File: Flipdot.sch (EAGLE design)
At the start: 20 parts, among them IC1 ULN2003, IC10 ULN2003, IC11 M74HC238, IC12 M74HC238, IC13 M74HC238, IC14 TD62783_AFWG, IC15 ULN2003, IC16 TD62783_AFWG, IC17 ULN2003, IC18 M74HC238, IC2 TD62783_AFWG, IC3 M74HC238, IC4 M74HC238, IC5 M74HC238, IC6 M74HC238, IC7 TD62783_AFWG, IC8 ULN2003, IC9 TD62783_AFWG, J1 HEADER

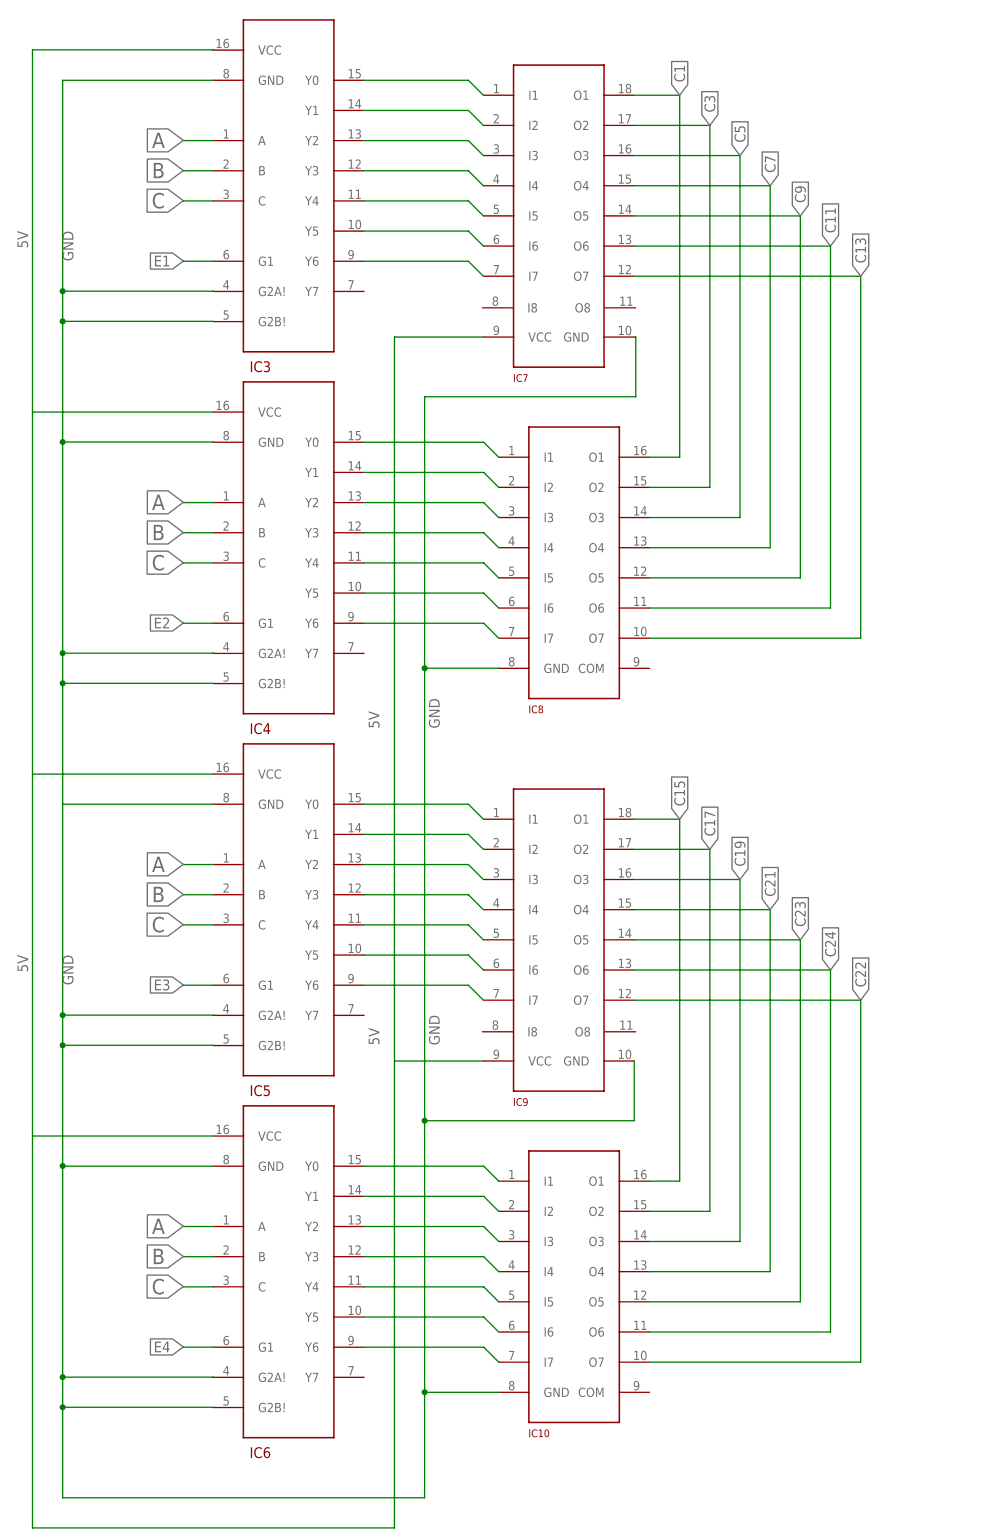
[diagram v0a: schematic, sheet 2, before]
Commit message: Finished
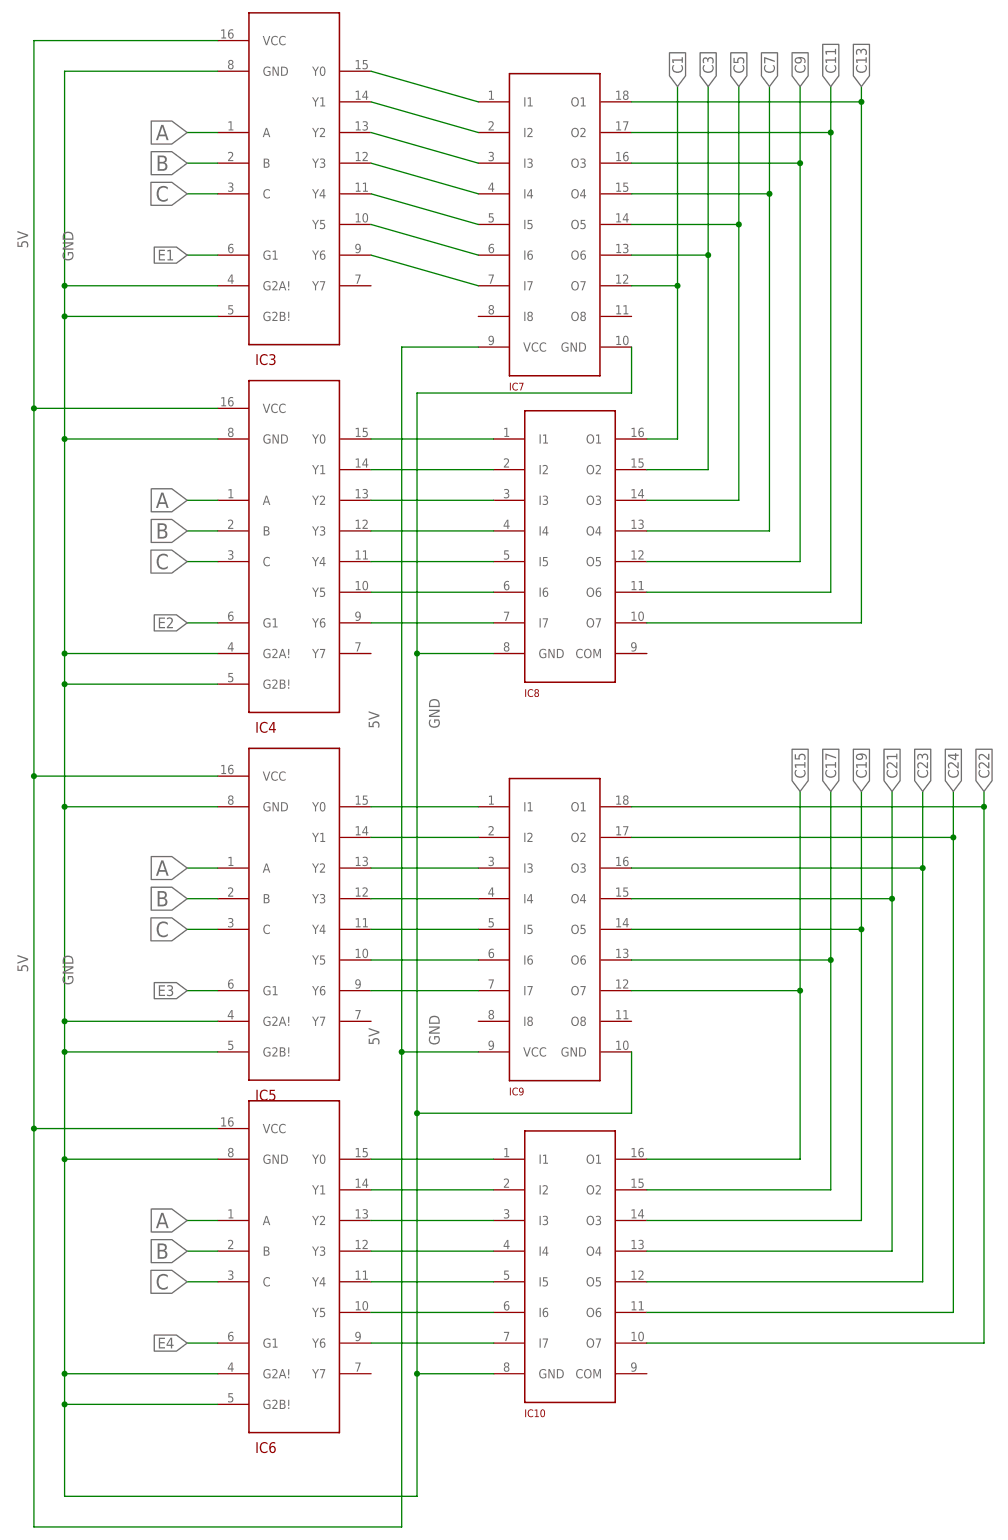
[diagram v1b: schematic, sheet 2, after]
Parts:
- removed MC1: SPARKFUN_PRO_MICRO, Flipdot:SPARKFUN_PRO_MICRO
- added IC19, IC20: M74HC238, Flipdot:M74HC238
- added MCU1: SPARKFUN_PRO_MICRO, Flipdot:SPARKFUN_PRO_MICRO
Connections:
- new net 12V: MCU1.RAW
- new net N$15: IC1.I1, IC19.Y1
- new net N$16: IC1.I2, IC19.Y2
- new net N$17: IC1.I3, IC19.Y3
- new net N$18: IC1.I4, IC19.Y4
- new net N$19: IC1.I5, IC19.Y5
- new net N$20: IC1.I6, IC19.Y6
- new net N$21: IC1.I7, IC19.Y7
- new net N$24: IC2.I1, IC20.Y1
- new net N$25: IC2.I2, IC20.Y2
- new net N$26: IC2.I3, IC20.Y3
- new net N$27: IC2.I4, IC20.Y4
- new net N$28: IC2.I5, IC20.Y5
- new net N$29: IC2.I6, IC20.Y6
- new net N$30: IC2.I7, IC20.Y7
- new net RA: IC19.A, IC20.A, MCU1.8
- new net RB: IC19.B, IC20.B, MCU1.*9
- new net RC: IC19.C, IC20.C, MCU1.*10
- new net RE: IC19.G1, IC20.G2A!, MCU1.A0
- net 5V: now also IC19.VCC, IC20.G1, IC20.VCC, MCU1.VCC
- net A: now also MCU1.2; no longer MC1.2
- net B: now also MCU1.*3; no longer MC1.*3
- net C: now also MCU1.4; no longer MC1.4
- net C1: now also IC7.O7; no longer IC7.O1
- net C10: now also IC14.O2; no longer IC14.O6
- net C11: now also IC7.O2; no longer IC7.O6
- net C12: now also IC14.O3; no longer IC14.O5
- net C13: now also IC7.O1; no longer IC7.O7
- net C15: now also IC9.O7; no longer IC9.O1
- net C16: now also IC14.O5; no longer IC14.O3
- net C17: now also IC9.O6; no longer IC9.O2
- net C18: now also IC14.O6; no longer IC14.O2
- net C19: now also IC9.O5; no longer IC9.O3
- net C2: now also IC16.O1; no longer IC16.O3
- net C20: now also IC14.O7; no longer IC14.O1
- net C22: now also IC9.O1; no longer IC9.O7
- net C23: now also IC9.O3; no longer IC9.O5
- net C24: now also IC9.O2; no longer IC9.O6
- net C3: now also IC7.O6; no longer IC7.O2
- net C5: now also IC7.O5; no longer IC7.O3
- net C6: now also IC16.O3; no longer IC16.O1
- net C8: now also IC14.O1; no longer IC14.O7
- net C9: now also IC7.O3; no longer IC7.O5
- net EA: now also MCU1.*5; no longer MC1.*5
- net EB: now also MCU1.*6; no longer MC1.*6
- net EC: now also MCU1.7; no longer MC1.7
- net GND: now also IC19.G2A!, IC19.G2B!, IC19.GND, IC20.G2B!, IC20.GND, MCU1.GND, MCU1.GND@1, MCU1.GND@2; no longer MC1.GND@2
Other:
- moved on the sheet: IC1, IC10, IC11, IC12, IC13, IC14, IC15, IC16, IC17, IC18, IC2, IC3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
